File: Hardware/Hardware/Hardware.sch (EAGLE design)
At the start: 9 parts, among them J1 1x10 HEADER "A", J2 1x10 HEADER "B", U1 MAX3232

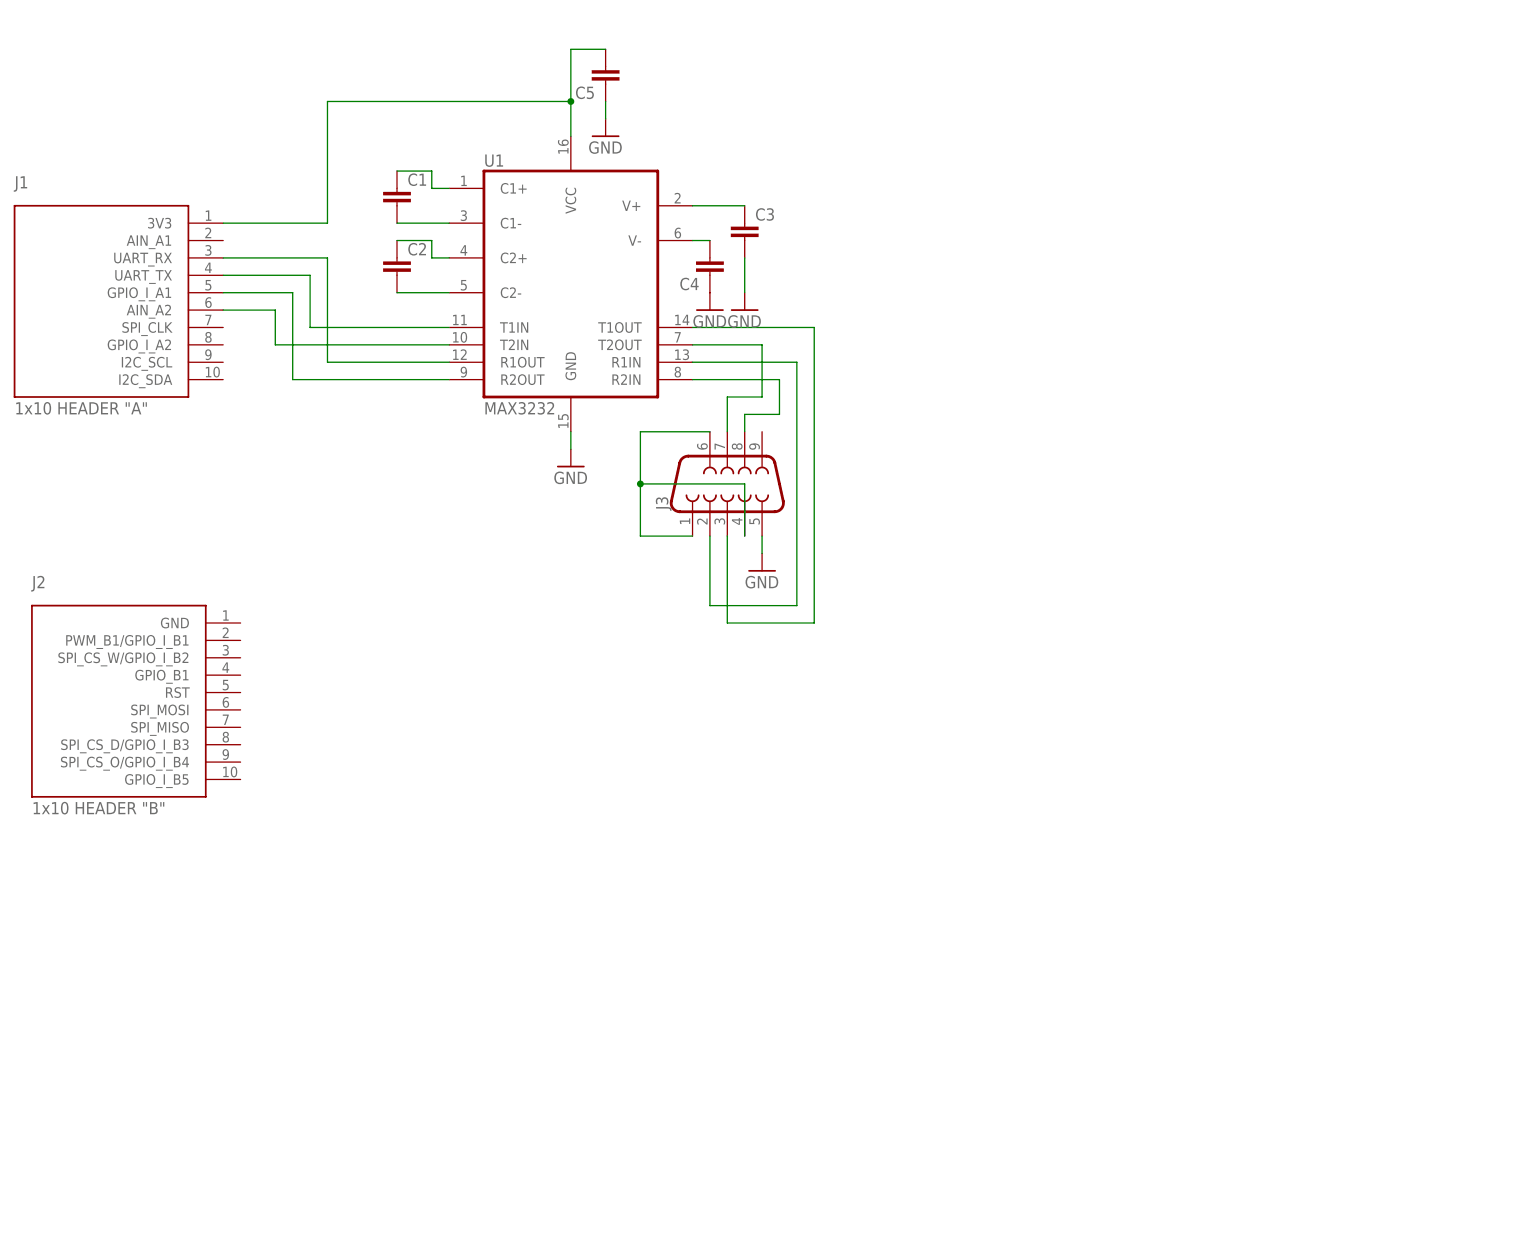
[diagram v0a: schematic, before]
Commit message: Merged the circuit diagrams
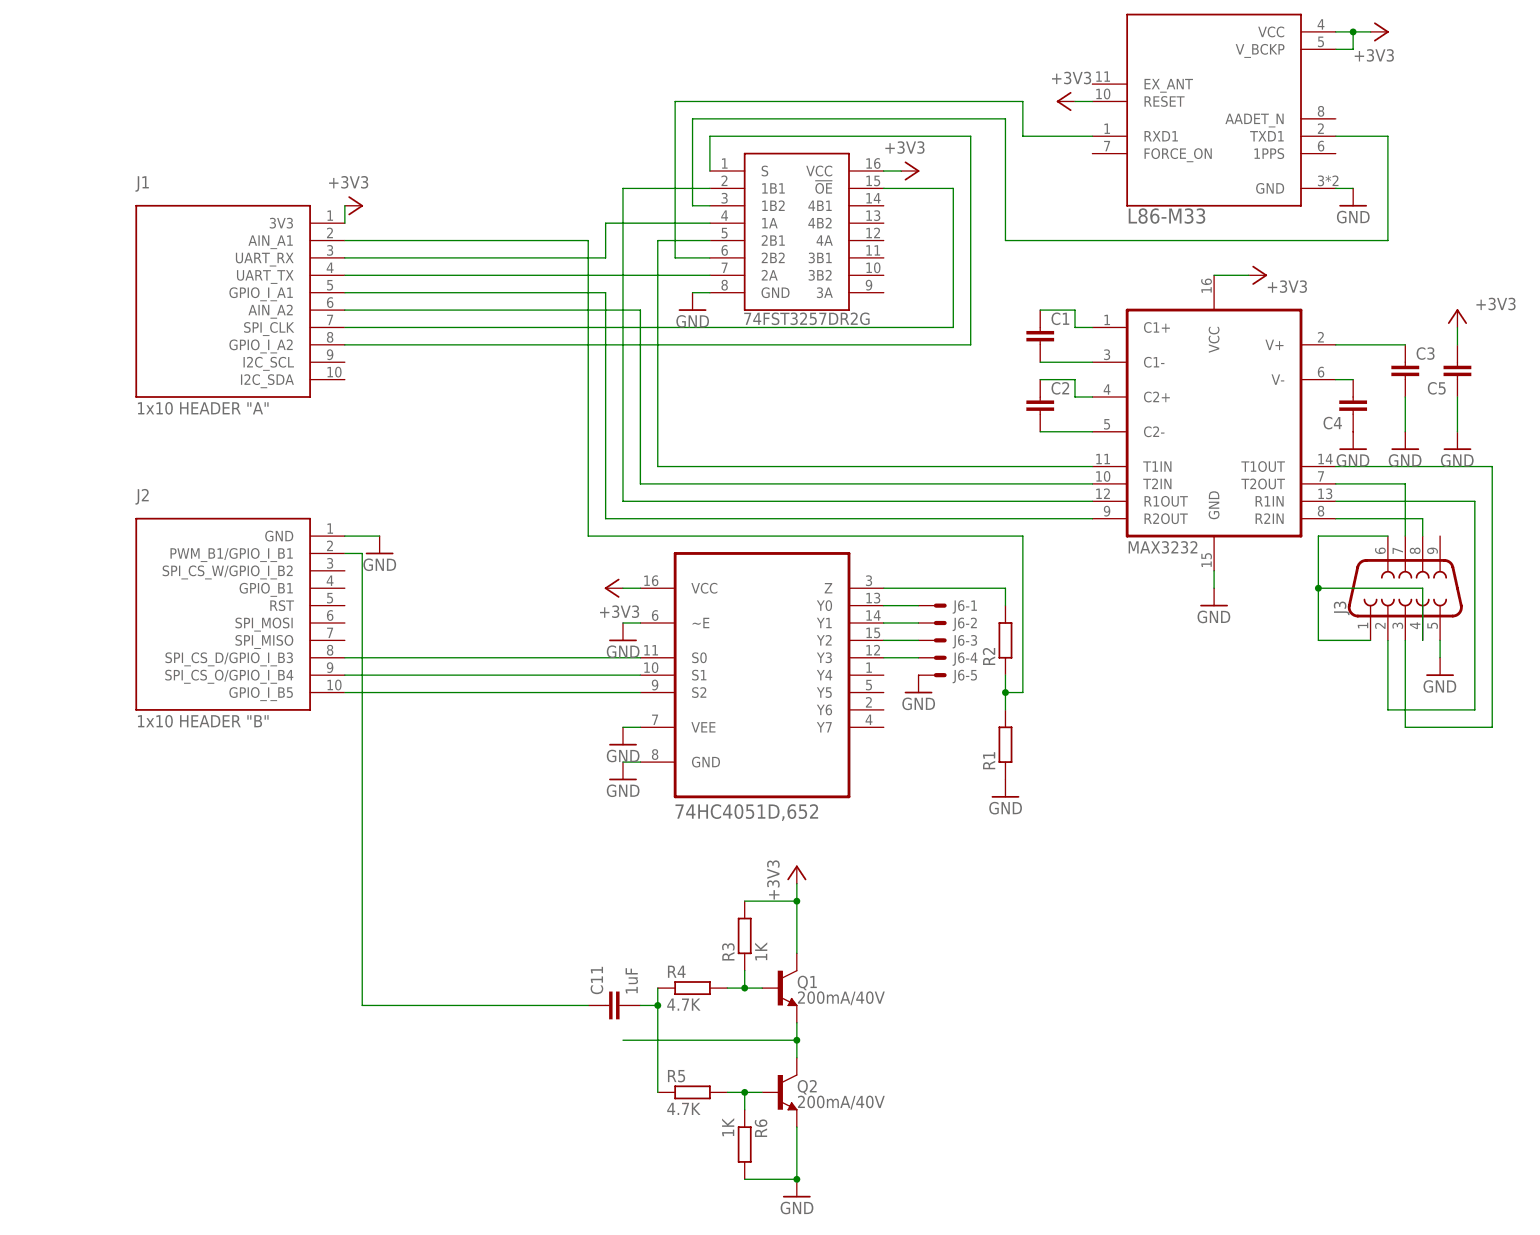
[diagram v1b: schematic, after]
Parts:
- added C11: 1uF, rcl:C-EU025-024X044
- added IC1: 74FST3257DR2G, 74FST3257DR2G:74FST3257DR2G
- added J6: 22-27-2051-05, con-molex:22-27-2051-05
- added Q1, Q2: 200mA/40V, SparkFun-DiscreteSemi:TRANS_NPN-2N3904
- added R1, R2: (no value), rcl:R-EU_0207/7
- added R3, R6: 1K, rcl:R-EU_0207/7
- added R4, R5: 4.7K, rcl:R-EU_0207/7
- added U2: L86-M33, L86-M33:L86-M33
- added U4: 74HC4051D,652, 74HC4051D_652:74HC4051D,652
- U1: device SparkFun-IC-Comms:MAX2323TSSOP -> SparkFun-IC-Comms:MAX2323SOIC16
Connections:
- removed net N$9 (its old number): J1.UART_TX, U1.T1IN
- new net +3V3: C5.2, IC1.VCC, J1.3V3, Q1.C, R3.2, U1.VCC, U2.RESET, U2.VCC, U2.V_BCKP, U4.VCC
- new net N$10: IC1.2B2, U2.RXD1
- new net N$11: IC1.1B1, U1.R1OUT
- new net N$17: IC1.2B1, U1.T1IN
- new net N$18: IC1.S, J1.GPIO_I_A2
- new net N$19: IC1.!OE, J1.SPI_CLK
- new net N$20: J6-1.S, U4.Y0
- new net N$22: J6-2.S, U4.Y1
- new net N$23: J6-3.S, U4.Y2
- new net N$24: J6-4.S, U4.Y3
- new net N$25: R2.2, U4.Z
- new net N$3: IC1.1A, J1.UART_RX
- new net N$47: J1.AIN_A1, R1.2, R2.1
- new net N$49: J2.SPI_CS_D/GPIO_I_B3, U4.S0
- new net N$50: J2.SPI_CS_O/GPIO_I_B4, U4.S1
- new net N$51: J2.GPIO_I_B5, U4.S2
- new net N$52: C11.2, R4.1, R5.1
- new net N$53: C11.1, J2.PWM_B1/GPIO_I_B1
- new net N$54: Q2.B, R5.2, R6.1
- new net N$55: Q1.B, R3.1, R4.2
- new net N$57: Q1.E, Q2.C
- net GND: now also IC1.GND, J2.GND, J6-5.S, Q2.E, R1.1, R6.2, U2.GND, U4.GND, U4.VEE, U4.~E
- net N$5: now also IC1.2A, J1.UART_TX; no longer C5.2, J1.3V3, U1.VCC
- net N$8: now also IC1.1B2, U2.TXD1; no longer J1.UART_RX, U1.R1OUT
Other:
- moved on the sheet: C1, C2, C3, C4, C5, J1, J2, J3
